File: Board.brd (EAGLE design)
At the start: 58.1 x 41.9 mm, 9 parts, among them IC1 317EMP

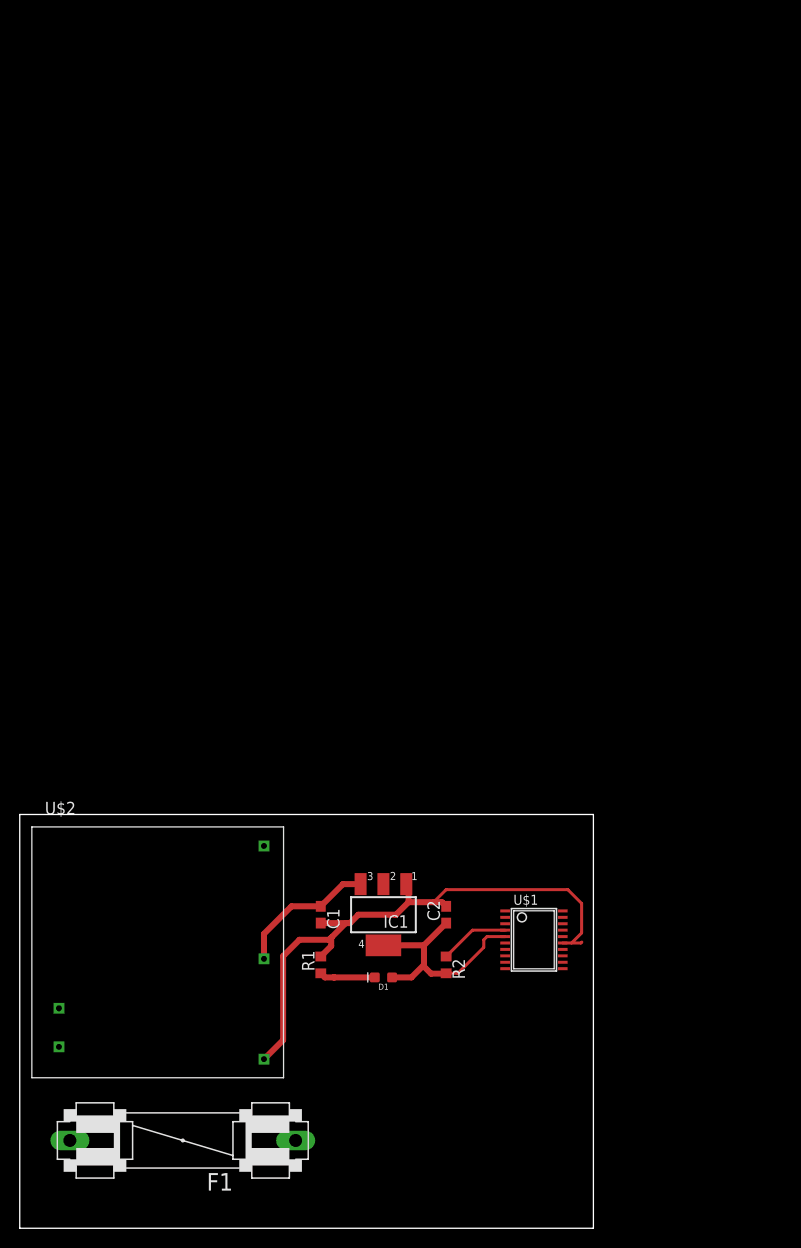
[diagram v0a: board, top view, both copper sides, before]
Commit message: preliminary board design
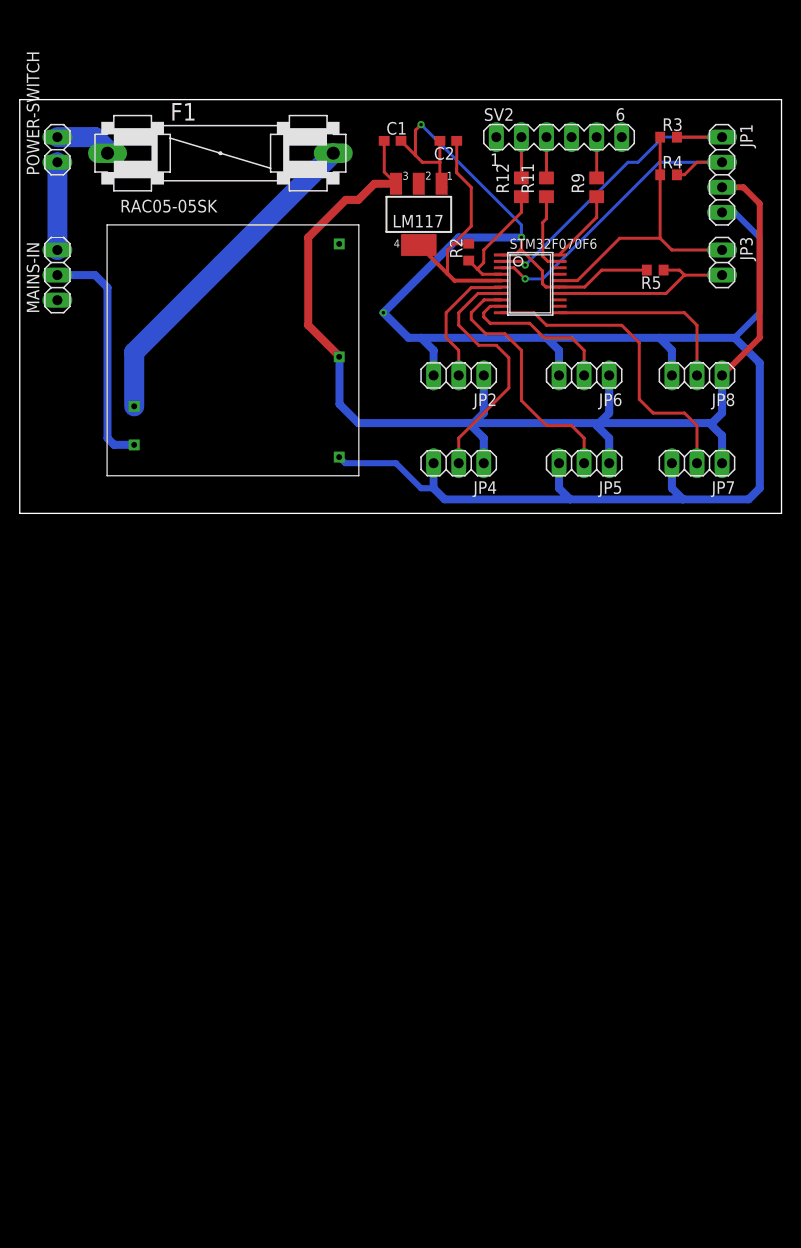
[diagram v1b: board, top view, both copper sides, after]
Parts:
- removed D1: GREEN, SparkFun-LED:LED-0603
- removed IC1: 317EMP, linear:SOT223
- removed R1: 200r, rcl:R0603
- removed U$1: STM32F07, chip:TSSOP20
- removed U$2: AC/DC-CONVERTER, Library:AC/DC-CONVERTER
- added JP1: (no value), pinhead:1X04
- added JP2, JP4, JP5, JP6, JP7, JP8, MAINS-IN: (no value), pinhead:1X03
- added JP3, POWER-SWITCH: (no value), pinhead:1X02
- added LM117: 317EMP, linear:SOT223
- added R11, R12, R9: 250, rcl:R0805
- added R3, R4: 3k3, rcl:R0603
- added R5: 1k5, rcl:R0603
- added RAC05-05SK: AC/DC-CONVERTER, Library:AC/DC-CONVERTER
- added STM32F070F6: (no value), SousVide Library:TSSOP20
- added SV2: (no value), con-lstb:MA06-1
- R2: value 3k -> 3k3
- moved F1 100.0 mm to (20.3, 108.9), turned to 0 degrees
- moved C1 78.7 mm to (37.8, 110.1), turned to 0 degrees
- moved C2 78.4 mm to (43.4, 110.1), turned to 180 degrees
- moved R2 72.2 mm to (45.5, 98.8), turned to 90 degrees
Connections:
- removed net N$1: D1.C, R1.1
- removed net N$3: U$1.16
- removed net N$6: R2.1, U$1.4
- new net EXTRA2: STM32F070F6.13
- new net EXTRA3: STM32F070F6.12
- new net GND: SV2.4
- new net N$19: R9.2, SV2.5
- new net N$21: R11.2, SV2.3
- new net N$22: R12.2, SV2.2
- new net N$7: MAINS-IN.3, POWER-SWITCH.1
- new net NRST: R12.1, R2.1, STM32F070F6.4
- new net PGND: MAINS-IN.1
- new net RELAY1: JP2.2, STM32F070F6.6
- new net RELAY2: JP4.2, STM32F070F6.7
- new net RELAY3: JP5.2, STM32F070F6.8
- new net RELAY4: JP6.2, STM32F070F6.9
- new net RELAY5: JP7.2, STM32F070F6.10
- new net RELAY6: JP8.2, STM32F070F6.11
- new net RX: STM32F070F6.18
- new net SCL: JP1.2, R4.2, STM32F070F6.3
- new net SDA: JP1.1, R3.2, STM32F070F6.2
- new net SWCLK: R9.1, STM32F070F6.20
- new net SWDIO: R11.1, STM32F070F6.19
- new net SWO: SV2.1
- new net TEMP-READ: JP3.2, R5.1, STM32F070F6.14
- new net TX: STM32F070F6.17
- net +3V3: now also JP3.1, LM117.4, R3.1, R4.1, STM32F070F6.16, STM32F070F6.5, SV2.6; no longer D1.A, IC1.4, U$1.5
- net +5V: now also JP1.3, JP2.1, JP4.1, JP5.1, JP6.1, JP7.1, JP8.1, LM117.3, RAC05-05SK.P$4; no longer IC1.3, U$2.P$4
- net PE: now also JP1.4, JP2.3, JP4.3, JP5.3, JP6.3, JP7.3, JP8.3, LM117.1, R5.2, RAC05-05SK.P$5, STM32F070F6.1, STM32F070F6.15; no longer IC1.1, R1.2, U$1.15, U$2.P$5
- net VAC(L): now also RAC05-05SK.P$1; no longer U$2.P$1
- net VAC(L)-INPUT: now also POWER-SWITCH.2
- net VAC(N): now also MAINS-IN.2, RAC05-05SK.P$2; no longer U$2.P$2
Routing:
- net PE: track 59.5 -> 202.7 mm, vias 0 -> 3
- net +5V: track 14.4 -> 125.9 mm
- net VAC(L): track 0.00 -> 34.0 mm
- net SCL: track 0.00 -> 32.8 mm, vias 0 -> 1
- net SDA: track 0.00 -> 32.4 mm, vias 0 -> 1
- net +3V3: track 23.7 -> 55.5 mm
- net RELAY5: track 0.00 -> 31.7 mm
- net RELAY3: track 0.00 -> 26.2 mm
- net RELAY2: track 0.00 -> 25.6 mm
- net VAC(N): track 0.00 -> 23.8 mm
- net TEMP-READ: track 0.00 -> 19.6 mm
- net RELAY6: track 0.00 -> 19.6 mm
- net RELAY4: track 0.00 -> 16.6 mm
- net RELAY1: track 0.00 -> 13.5 mm
- net NRST: track 0.00 -> 13.1 mm
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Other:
- board size 58.1 x 41.9 mm -> 77.1 x 41.9 mm
